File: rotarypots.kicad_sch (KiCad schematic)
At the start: 20 parts, among them U1 CD74HC4067M96, U2 CD74HC4067M96

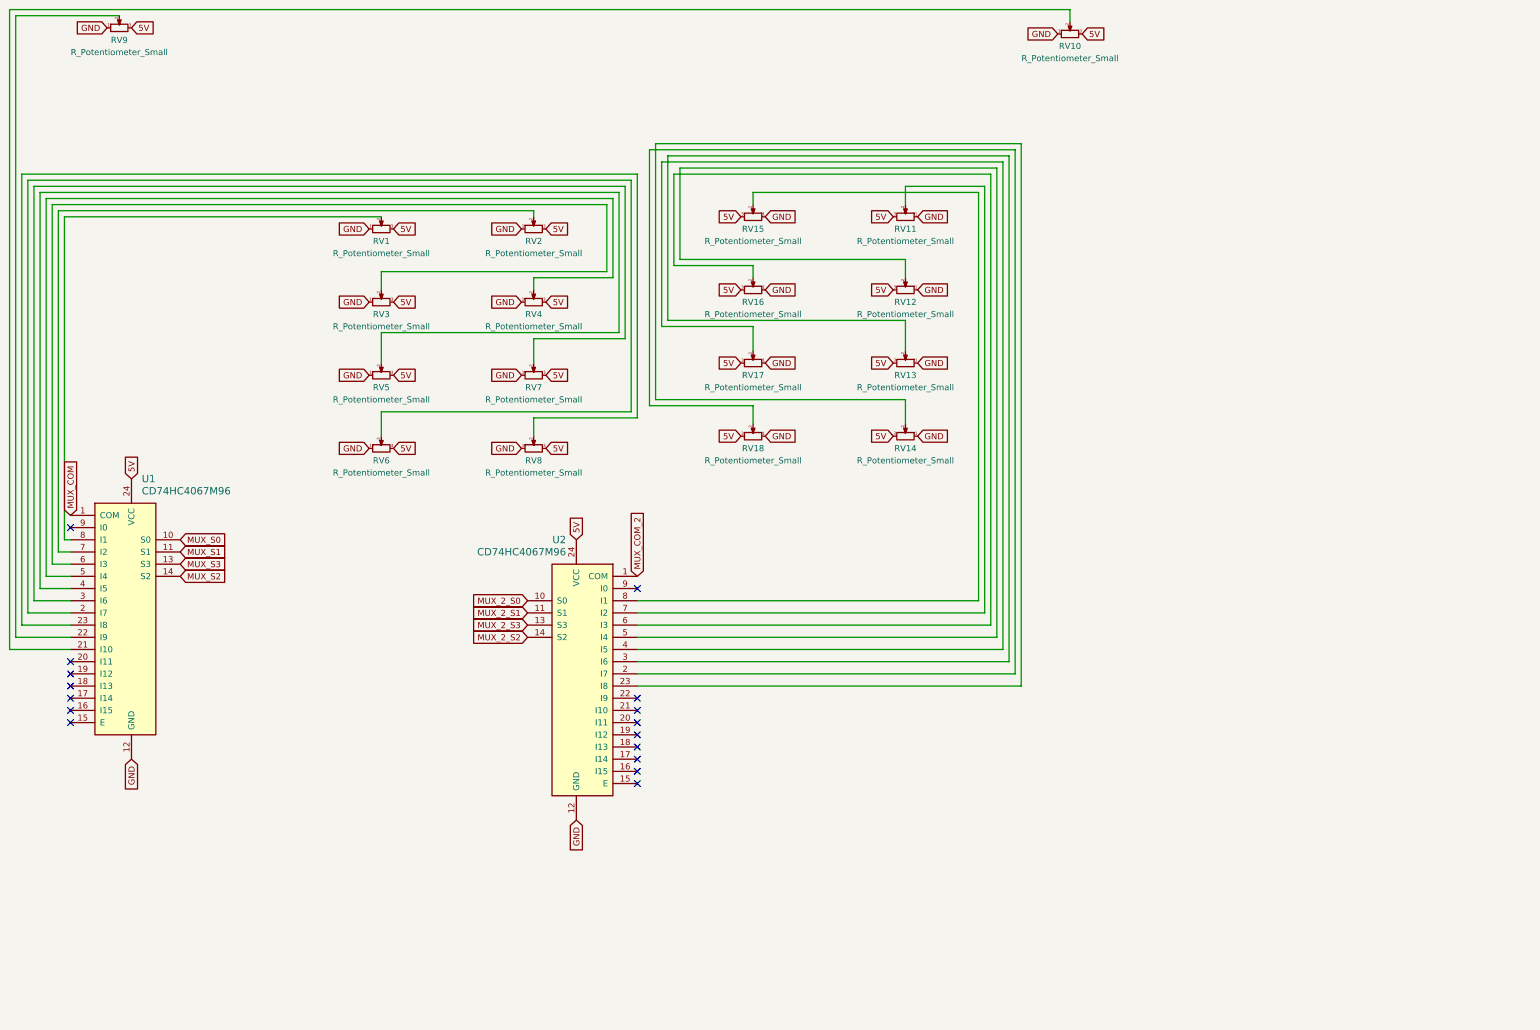
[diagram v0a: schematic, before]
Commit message: Add files via upload
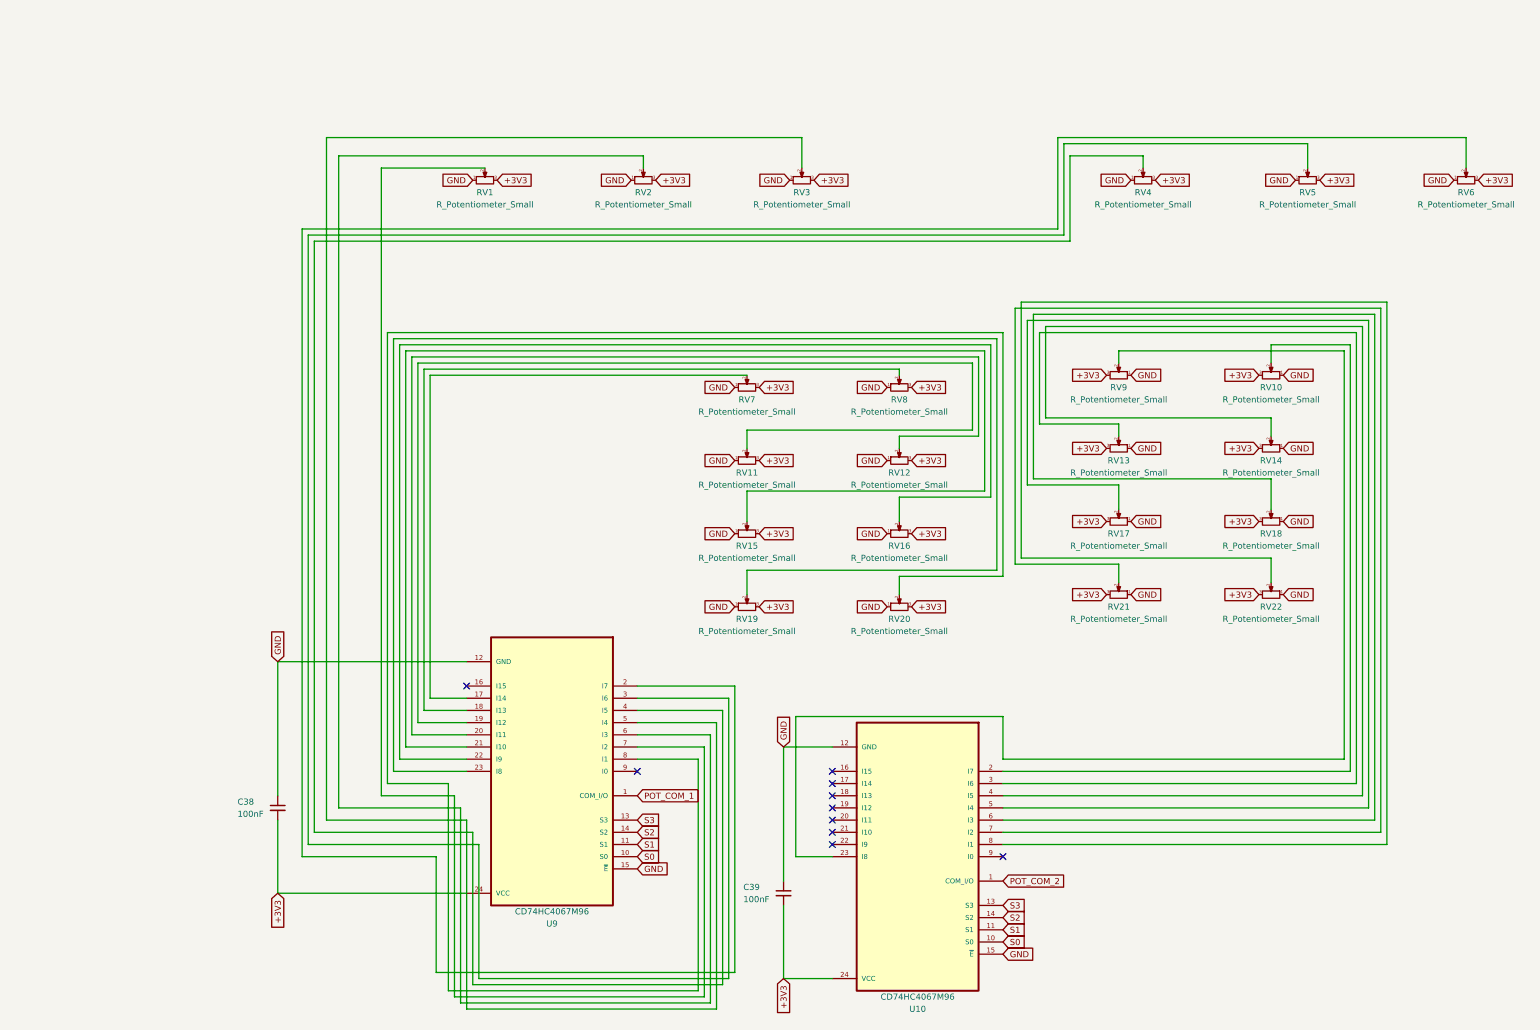
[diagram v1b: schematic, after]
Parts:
- removed U1, U2: CD74HC4067M96, digikey-footprints:SOIC-24_W7.50mm, symbol dk_Interface-Analog-Switches-Multiplexers-Demultiplexers:CD74HC4067M96
- added C38, C39: 100nF, Capacitor_SMD:C_0603_1608Metric, symbol Device:C_Small
- added RV3, RV4, RV5, RV6: R_Potentiometer_Small, rotary_pots_eq:RK09D1130C3W_using_RK09D1130009_footprint_ALPS, symbol Device:R_Potentiometer_Small
- added U10, U9: CD74HC4067M96, CD74HC4067M96:SOIC127P1030X265-24N, symbol CD74HC4067M96:CD74HC4067M96
- RV1: renamed from RV9; footprint (none) -> rotary_pots_eq:RK09D1130C3W_using_RK09D1130009_footprint_ALPS
- RV10: renamed from RV11; footprint (none) -> rotary_pots_eq:RK09D1130C3W_using_RK09D1130009_footprint_ALPS
- RV11: renamed from RV3; footprint (none) -> rotary_pots_eq:RK09D1130C3W_using_RK09D1130009_footprint_ALPS
- RV12: renamed from RV4; footprint (none) -> rotary_pots_eq:RK09D1130C3W_using_RK09D1130009_footprint_ALPS
- RV13: renamed from RV16; footprint (none) -> rotary_pots_eq:RK09D1130C3W_using_RK09D1130009_footprint_ALPS
- RV14: renamed from RV12; footprint (none) -> rotary_pots_eq:RK09D1130C3W_using_RK09D1130009_footprint_ALPS
- RV15: renamed from RV5; footprint (none) -> rotary_pots_eq:RK09D1130C3W_using_RK09D1130009_footprint_ALPS
- RV16: renamed from RV7; footprint (none) -> rotary_pots_eq:RK09D1130C3W_using_RK09D1130009_footprint_ALPS
- RV17: footprint (none) -> rotary_pots_eq:RK09D1130C3W_using_RK09D1130009_footprint_ALPS
- RV18: renamed from RV13; footprint (none) -> rotary_pots_eq:RK09D1130C3W_using_RK09D1130009_footprint_ALPS
- RV19: renamed from RV6; footprint (none) -> rotary_pots_eq:RK09D1130C3W_using_RK09D1130009_footprint_ALPS
- RV2: renamed from RV10; footprint (none) -> rotary_pots_eq:RK09D1130C3W_using_RK09D1130009_footprint_ALPS
- RV20: renamed from RV8; footprint (none) -> rotary_pots_eq:RK09D1130C3W_using_RK09D1130009_footprint_ALPS
- RV21: renamed from RV18; footprint (none) -> rotary_pots_eq:RK09D1130C3W_using_RK09D1130009_footprint_ALPS
- RV22: renamed from RV14; footprint (none) -> rotary_pots_eq:RK09D1130C3W_using_RK09D1130009_footprint_ALPS
- RV7: renamed from RV1; footprint (none) -> rotary_pots_eq:RK09D1130C3W_using_RK09D1130009_footprint_ALPS
- RV8: renamed from RV2; footprint (none) -> rotary_pots_eq:RK09D1130C3W_using_RK09D1130009_footprint_ALPS
- RV9: renamed from RV15; footprint (none) -> rotary_pots_eq:RK09D1130C3W_using_RK09D1130009_footprint_ALPS
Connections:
- net GND: now also C38.1, C39.1, RV3.1, RV4.1, RV5.1, RV6.1, U10.12 (GND), U10.15 (~{E}), U9.12 (GND), U9.15 (~{E})
- net at RV20.2: now also U9.8 (I1)
- net at RV7.2: now also U9.17 (I14)
- net at RV19.2: now also U9.23 (I8)
- net at RV2.2: now also U9.6 (I3)
- net at RV1.2: now also U9.7 (I2)
- net at RV16.2: now also U9.22 (I9)
- net at RV15.2: now also U9.21 (I10)
- net at RV12.2: now also U9.20 (I11)
- net at RV11.2: now also U9.19 (I12)
- net at RV8.2: now also U9.18 (I13)
- net at RV17.2: now also U10.5 (I4)
- net at RV21.2: now also U10.7 (I2)
- net at RV22.2: now also U10.8 (I1)
- net at RV18.2: now also U10.6 (I3)
- net at RV14.2: now also U10.4 (I5)
- net at RV13.2: now also U10.3 (I6)
- net at RV10.2: now also U10.2 (I7)
- net at RV9.2: now also U10.23 (I8)
- net 5V renamed +3V3
- net +3V3: now also C38.2, C39.2, RV3.3, RV4.3, RV5.3, RV6.3, U10.24 (VCC), U9.24 (VCC)
- new net: RV4.2, U9.4 (I5)
- new net: RV6.2, U9.2 (I7)
- new net: RV5.2, U9.3 (I6)
- new net: RV3.2, U9.5 (I4)
- new net POT_COM_1: U9.1 (COM_I/O)
- new net POT_COM_2: U10.1 (COM_I/O)
- new net S0: U10.10 (S0), U9.10 (S0)
- new net S1: U10.11 (S1), U9.11 (S1)
- new net S2: U10.14 (S2), U9.14 (S2)
- new net S3: U10.13 (S3), U9.13 (S3)
- no-connect marks 16 -> 10
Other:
- company: (none) -> Alex G
- title: (none) -> @opensourcedj on twitter
- moved on the sheet: RV1, RV10, RV11, RV12, RV13, RV14, RV15, RV16, RV17, RV18, RV19, RV2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
